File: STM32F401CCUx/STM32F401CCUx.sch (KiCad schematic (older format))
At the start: 57 parts, among them J1 Conn_01x04, J2 Power_Conn, J3 SWD, J4 USB_C_Receptacle_USB2.0, Q1 AO3401A, SW1 SW_SPDT, U1 MSM38A2718Z9BM3, U2 EUP3458, U3 LM321, U4 STM32F401CCUx, U5 USBLC6-2SC6, Y1 25MHz

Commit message: PCB
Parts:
- C1, C13, C16, C2, C3, C4, C5, C6: footprint (none) -> Capacitor_SMD:C_0402_1005Metric
- C10, C11, C12, C9: footprint (none) -> Capacitor_SMD:C_0603_1608Metric_Pad1.05x0.95mm_HandSolder
- C14: footprint (none) -> Capacitor_SMD:CP_Elec_4x5.7
- C15: value 10p -> 10p C335976; footprint (none) -> Capacitor_SMD:C_0402_1005Metric
- C7: footprint (none) -> Capacitor_SMD:C_0603_1608Metric
- C8: footprint (none) -> Capacitor_SMD:CP_Elec_4x5.3
- D1, D3: footprint (none) -> Diode_SMD:D_SOD-123
- D4, D5: footprint (none) -> Diode_SMD:D_0402_1005Metric
- F1: footprint (none) -> Fuse:Fuseholder_Blade_Mini_Keystone_3568
- FB1, FB2: footprint (none) -> Resistor_SMD:R_0805_2012Metric_Pad1.15x1.40mm_HandSolder
- J1: footprint (none) -> Connector_PinHeader_2.54mm:PinHeader_1x04_P2.54mm_Horizontal
- J2: footprint (none) -> Connector_BarrelJack:BarrelJack_Horizontal
- J3: footprint (none) -> Connector_PinHeader_2.54mm:PinHeader_2x05_P2.54mm_Horizontal
- J4: footprint (none) -> Connector_USB:USB_C_Receptacle_HRO_TYPE-C-31-M-12; symbol Connector:USB_C_Receptacle_USB2.0 -> STM32F401CCUx-rescue:USB_C_Receptacle_USB2.0-Connector
- L1, L2: footprint Inductor_SMD:L_1206_3216Metric_Pad1.22x1.90mm_HandSolder -> Inductor_SMD:L_1206_3216Metric
- R1, R2, R5, R6, R7: footprint Resistor_SMD:R_1206_3216Metric_Pad1.30x1.75mm_HandSolder -> Resistor_SMD:R_1206_3216Metric
- R10, R11, R12, R13, R14, R15, R16, R17, R18, R3, R4, R8, R9: footprint Resistor_SMD:R_0805_2012Metric_Pad1.20x1.40mm_HandSolder -> Resistor_SMD:R_0805_2012Metric
- R19: footprint Resistor_SMD:R_0402_1005Metric_Pad0.72x0.64mm_HandSolder -> Resistor_SMD:R_0402_1005Metric
- U1: footprint (none) -> MEMS:MEMS38A
- U5: symbol Power_Protection:USBLC6-2SC6 -> STM32F401CCUx-rescue:USBLC6-2SC6-Power_Protection
- Y1: footprint (none) -> Crystal:Crystal_SMD_3225-4Pin_3.2x2.5mm_HandSoldering

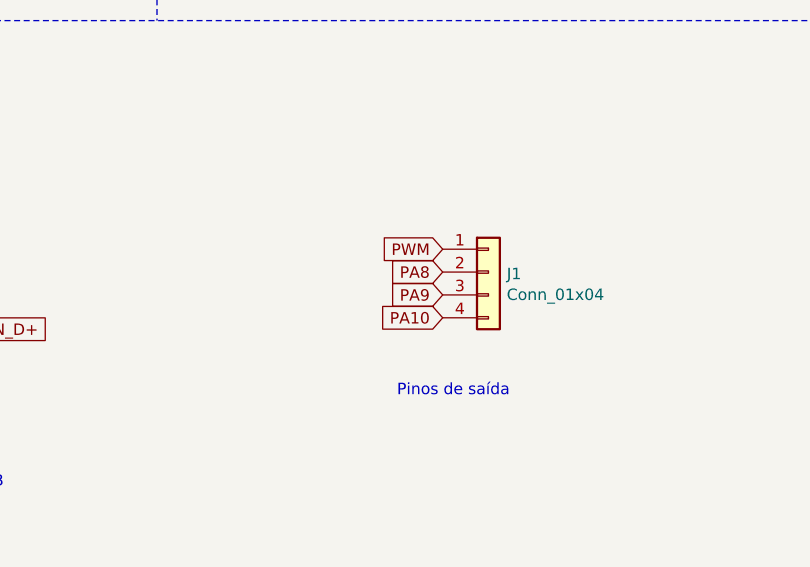
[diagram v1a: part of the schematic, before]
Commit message: Updated PCB
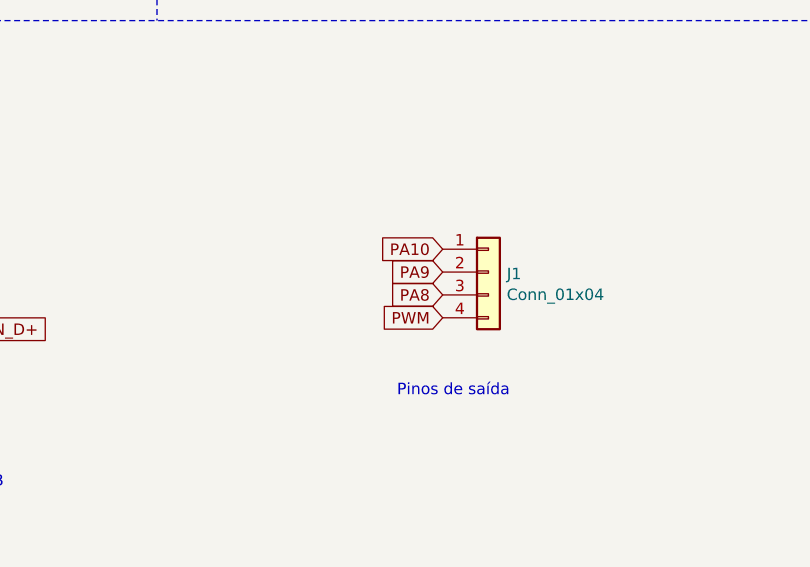
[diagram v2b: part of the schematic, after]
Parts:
- F1: footprint Fuse:Fuseholder_Blade_Mini_Keystone_3568 -> Fuse_holder:FUSE-TH_L22.6-W9.0
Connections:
- net PA10: now also J1.1 (Pin_1); no longer J1.4 (Pin_4)
- net PA8: now also J1.3 (Pin_3); no longer J1.2 (Pin_2)
- net PA9: now also J1.2 (Pin_2); no longer J1.3 (Pin_3)
- net PWM: now also J1.4 (Pin_4); no longer J1.1 (Pin_1)
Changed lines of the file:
@@
 F 0 "F1" V 925 1350 50  0000 C CNN
 F 1 "250mA" V 1016 1350 50  0000 C CNN
-F 2 "Fuse:Fuseholder_Blade_Mini_Keystone_3568" H 1200 1150 50  0001 L CNN
+F 2 "Fuse_holder:FUSE-TH_L22.6-W9.0" H 1200 1150 50  0001 L CNN
 F 3 "~" H 1150 1350 50  0001 C CNN
 	1    1150 1350
@@
 	1    0    0    -1
 $EndComp
+Text GLabel 9850 8050 0    50   Input ~ 0
+PA8
 Text GLabel 9850 7950 0    50   Input ~ 0
-PA8
-Text GLabel 9850 8050 0    50   Input ~ 0
 PA9
+Text GLabel 9850 7850 0    50   Input ~ 0
+PA10
 Text GLabel 9850 8150 0    50   Input ~ 0
-PA10
-Text GLabel 9850 7850 0    50   Input ~ 0
 PWM
 $Comp
